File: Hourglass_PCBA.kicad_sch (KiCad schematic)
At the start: 0 parts

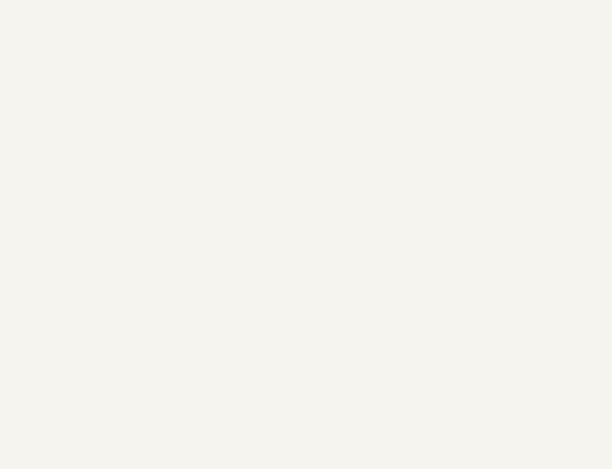
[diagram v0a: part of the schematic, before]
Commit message: Progress commit. Added MCU + IMU.
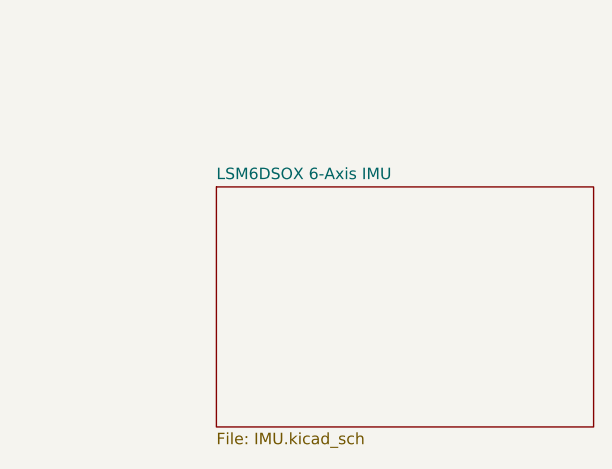
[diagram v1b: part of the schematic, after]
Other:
- added sheet LSM6DSOX 6-Axis IMU (IMU.kicad_sch)
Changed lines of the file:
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@@
+		)
+	)
+	(sheet
+		(at 121.92 87.63)
+		(size 41.91 26.67)
+		(fields_autoplaced yes)
+		(stroke
+			(width 0.1524)
+			(type solid)
+		)
+		(fill
+			(color 0 0 0 0.0000)
+		)
+		(property "Sheetname" "LSM6DSOX 6-Axis IMU"
+			(at 121.92 86.9184 0)
+			(effects
+				(font
+					(size 1.27 1.27)
+				)
+				(justify left bottom)
+			)
+		)
+		(property "Sheetfile" "IMU.kicad_sch"
+			(at 121.92 114.8846 0)
+			(effects
+				(font
+					(size 1.27 1.27)
+				)
+				(justify left top)
+			)
+		)
+		(instances
+			(project "Hourglass_PCBA"
+				(path "/a75630d2-15a7-42bc-8ce0-7846cbd1da6b"
+					(page "6")
+				)
+			)
 		)
 	)
